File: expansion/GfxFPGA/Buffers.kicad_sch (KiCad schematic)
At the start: 17 parts, among them U203 SN74LVC8T245PWR, U204 SN74LVC8T245PWR, U205 SN74LVC8T245PWR, U206 SN74LVC8T245PWR

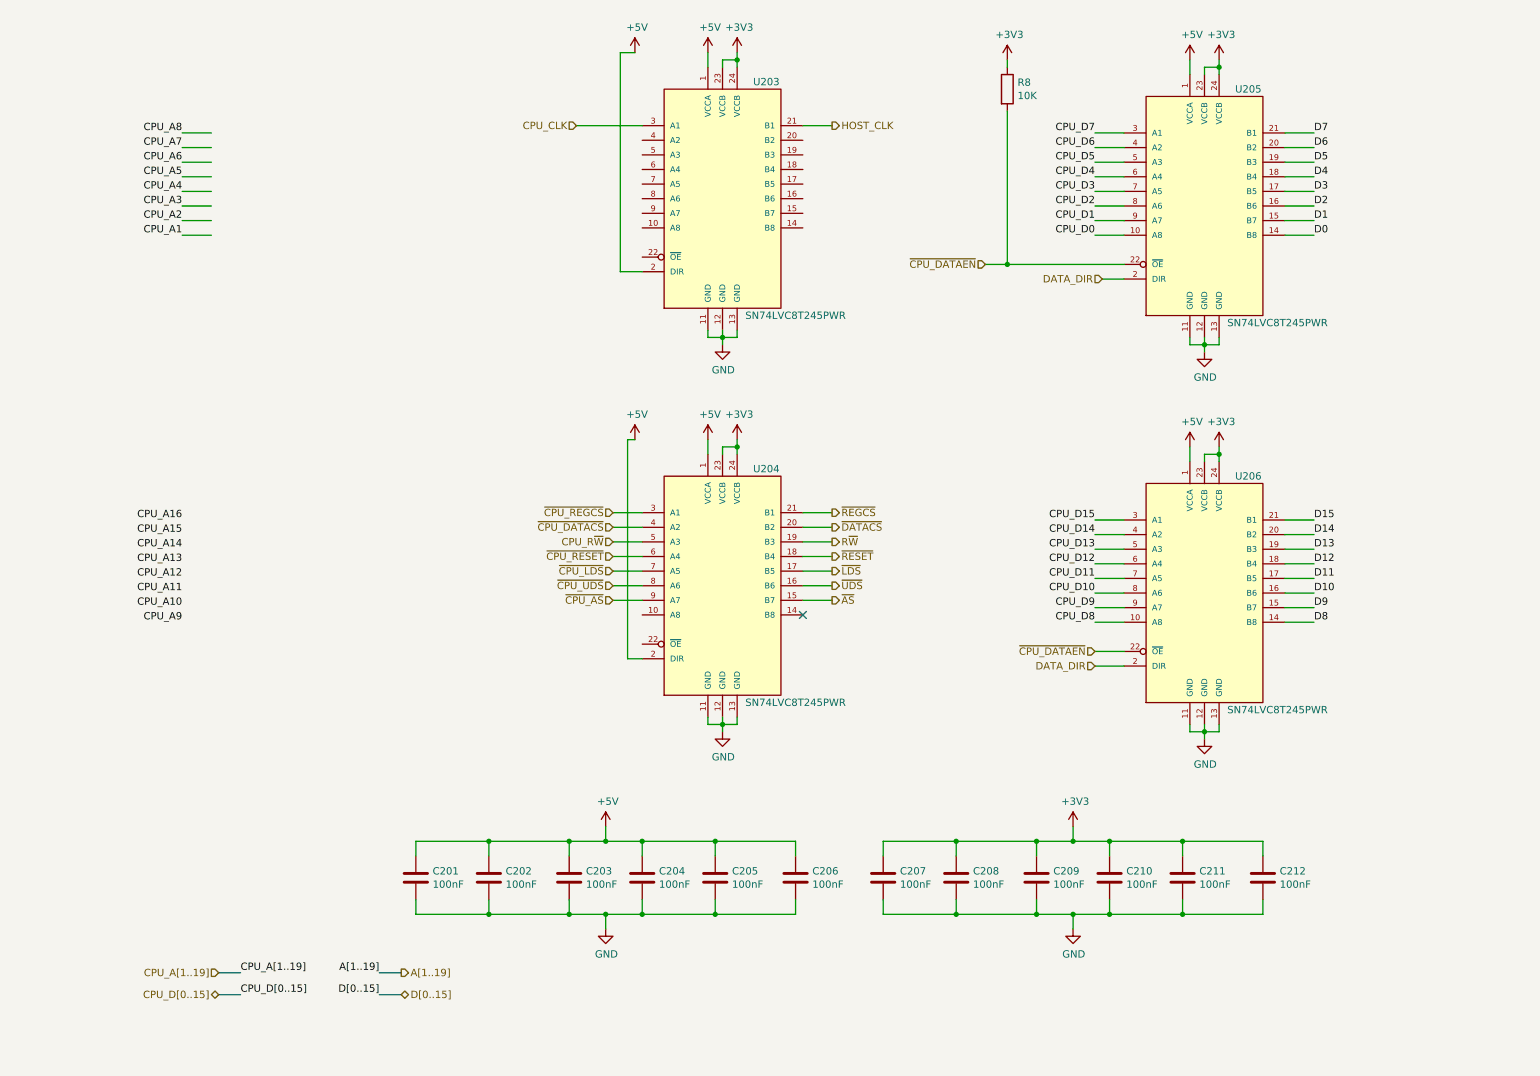
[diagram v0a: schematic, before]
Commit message: WOrking on VGA card
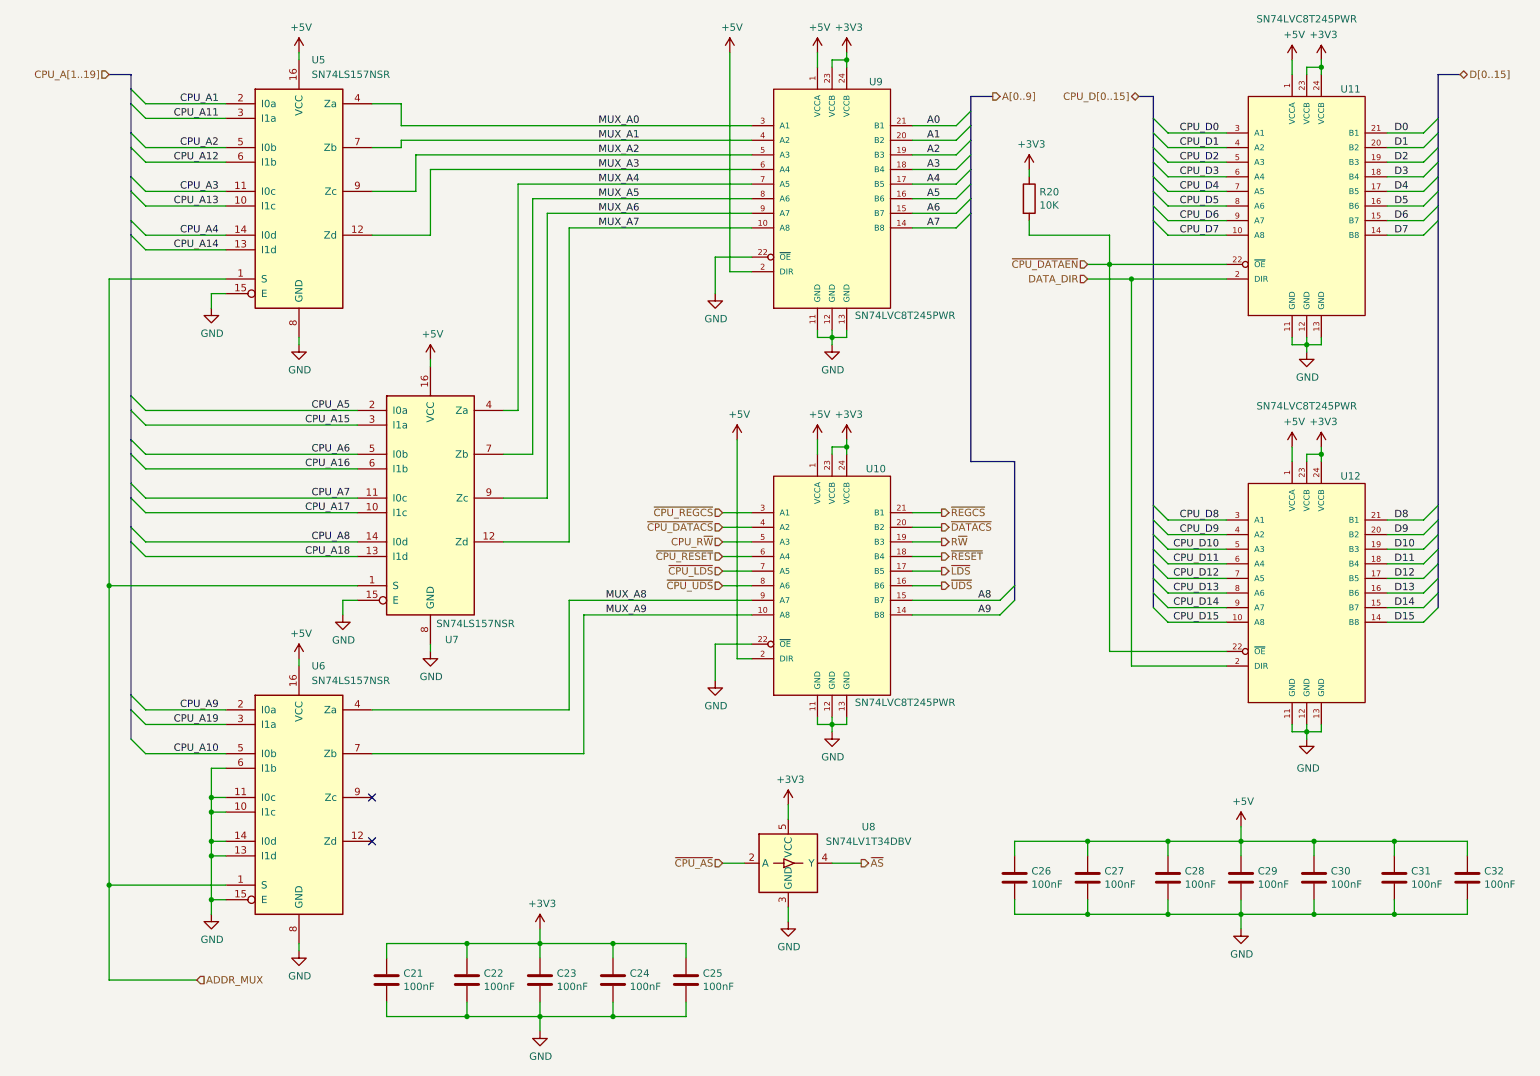
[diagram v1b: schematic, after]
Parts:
- removed C212: 100nF, Capacitor_SMD:C_0805_2012Metric, symbol Device:C
- added C25: 100nF, Capacitor_SMD:C_0805_2012Metric, symbol Device:C
- added U5, U6, U7: SN74LS157NSR, Package_SO:SO-16_5.3x10.2mm_P1.27mm, symbol 74xx:74LS157
- added U8: SN74LV1T34DBV, Package_TO_SOT_SMD:SOT-23-5, symbol Logic_LevelTranslator:SN74LV1T34DBV
- renumbered C208 to C21, C209 to C22, C210 to C23, C211 to C24, C201 to C26, C202 to C27, C203 to C28, C204 to C29, C205 to C30, C206 to C31, C207 to C32, R8 to R20, U204 to U10, U205 to U11, U206 to U12, U203 to U9
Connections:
- net +3V3: now also C25.1, U8.5 (VCC); no longer C32.1
- net +5V: now also C32.1, U5.16 (VCC), U6.16 (VCC), U7.16 (VCC)
- net CPU_A1: now also U5.2 (I0a)
- net CPU_A10: now also U6.5 (I0b)
- net CPU_A11: now also U5.3 (I1a)
- net CPU_A12: now also U5.6 (I1b)
- net CPU_A13: now also U5.10 (I1c)
- net CPU_A14: now also U5.13 (I1d)
- net CPU_A15: now also U7.3 (I1a)
- net CPU_A16: now also U7.6 (I1b)
- net CPU_A2: now also U5.5 (I0b)
- net CPU_A3: now also U5.11 (I0c)
- net CPU_A4: now also U5.14 (I0d)
- net CPU_A5: now also U7.2 (I0a)
- net CPU_A6: now also U7.5 (I0b)
- net CPU_A7: now also U7.11 (I0c)
- net CPU_A8: now also U7.14 (I0d)
- net CPU_A9: now also U6.2 (I0a)
- net CPU_D0: now also U11.3 (A1); no longer U11.10 (A8)
- net CPU_D1: now also U11.4 (A2); no longer U11.9 (A7)
- net CPU_D10: now also U12.5 (A3); no longer U12.8 (A6)
- net CPU_D11: now also U12.6 (A4); no longer U12.7 (A5)
- net CPU_D12: now also U12.7 (A5); no longer U12.6 (A4)
- net CPU_D13: now also U12.8 (A6); no longer U12.5 (A3)
- net CPU_D14: now also U12.9 (A7); no longer U12.4 (A2)
- net CPU_D15: now also U12.10 (A8); no longer U12.3 (A1)
- net CPU_D2: now also U11.5 (A3); no longer U11.8 (A6)
- net CPU_D3: now also U11.6 (A4); no longer U11.7 (A5)
- net CPU_D4: now also U11.7 (A5); no longer U11.6 (A4)
- net CPU_D5: now also U11.8 (A6); no longer U11.5 (A3)
- net CPU_D6: now also U11.9 (A7); no longer U11.4 (A2)
- net CPU_D7: now also U11.10 (A8); no longer U11.3 (A1)
- net CPU_D8: now also U12.3 (A1); no longer U12.10 (A8)
- net CPU_D9: now also U12.4 (A2); no longer U12.9 (A7)
- net D0: now also U11.21 (B1); no longer U11.14 (B8)
- net D1: now also U11.20 (B2); no longer U11.15 (B7)
- net D10: now also U12.19 (B3); no longer U12.16 (B6)
- net D11: now also U12.18 (B4); no longer U12.17 (B5)
- net D12: now also U12.17 (B5); no longer U12.18 (B4)
- net D13: now also U12.16 (B6); no longer U12.19 (B3)
- net D14: now also U12.15 (B7); no longer U12.20 (B2)
- net D15: now also U12.14 (B8); no longer U12.21 (B1)
- net D2: now also U11.19 (B3); no longer U11.16 (B6)
- net D3: now also U11.18 (B4); no longer U11.17 (B5)
- net D4: now also U11.17 (B5); no longer U11.18 (B4)
- net D5: now also U11.16 (B6); no longer U11.19 (B3)
- net D6: now also U11.15 (B7); no longer U11.20 (B2)
- net D7: now also U11.14 (B8); no longer U11.21 (B1)
- net D8: now also U12.21 (B1); no longer U12.14 (B8)
- net D9: now also U12.20 (B2); no longer U12.15 (B7)
- net GND: now also U10.22 (~{OE}), U9.22 (~{OE}), C25.2, U5.15 (E), U5.8 (GND), U6.10 (I1c), U6.11 (I0c), U6.13 (I1d), U6.14 (I0d), U6.15 (E), U6.6 (I1b), U6.8 (GND), U7.15 (E), U7.8 (GND), U8.3 (GND)
- net ~{AS}: now also U8.4 (Y); no longer U10.15 (B7)
- net ~{CPU_AS}: now also U8.2 (A); no longer U10.9 (A7)
- net MUX_A7: now reaches U9.10 (A8)
- net MUX_A7: now also U7.12 (Zd)
- net A7: now reaches U9.14 (B8)
- net A6: now reaches U9.15 (B7)
- net A5: now reaches U9.16 (B6)
- net A4: now reaches U9.17 (B5)
- net A3: now reaches U9.18 (B4)
- net A2: now reaches U9.19 (B3)
- net A1: now reaches U9.20 (B2)
- net MUX_A1: now reaches U9.4 (A2)
- net MUX_A1: now also U5.7 (Zb)
- net MUX_A2: now reaches U9.5 (A3)
- net MUX_A2: now also U5.9 (Zc)
- net MUX_A3: now reaches U9.6 (A4)
- net MUX_A3: now also U5.12 (Zd)
- net MUX_A4: now reaches U9.7 (A5)
- net MUX_A4: now also U7.4 (Za)
- net MUX_A5: now reaches U9.8 (A6)
- net MUX_A5: now also U7.7 (Zb)
- net MUX_A6: now reaches U9.9 (A7)
- net MUX_A6: now also U7.9 (Zc)
- net MUX_A9: now reaches U10.10 (A8)
- net MUX_A9: now also U6.7 (Zb)
- net A9: now reaches U10.14 (B8)
- net CPU_CLK renamed MUX_A0
- net MUX_A0: now also U5.4 (Za)
- net HOST_CLK renamed A0
- new net A8: U10.15 (B7)
- new net ADDR_MUX: U5.1 (S), U6.1 (S), U7.1 (S)
- new net CPU_A17: U7.10 (I1c)
- new net CPU_A18: U7.13 (I1d)
- new net CPU_A19: U6.3 (I1a)
- new net MUX_A8: U10.9 (A7), U6.4 (Za)
- no-connect marks 1 -> 2
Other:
- moved on the sheet: C21, C22, C23, C24, C26, C27, C28, C29, C30, C31, C32, R20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
